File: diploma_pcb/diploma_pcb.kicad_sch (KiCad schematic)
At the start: 15 parts, among them Q1 2SC3356, Q3 2SC3356

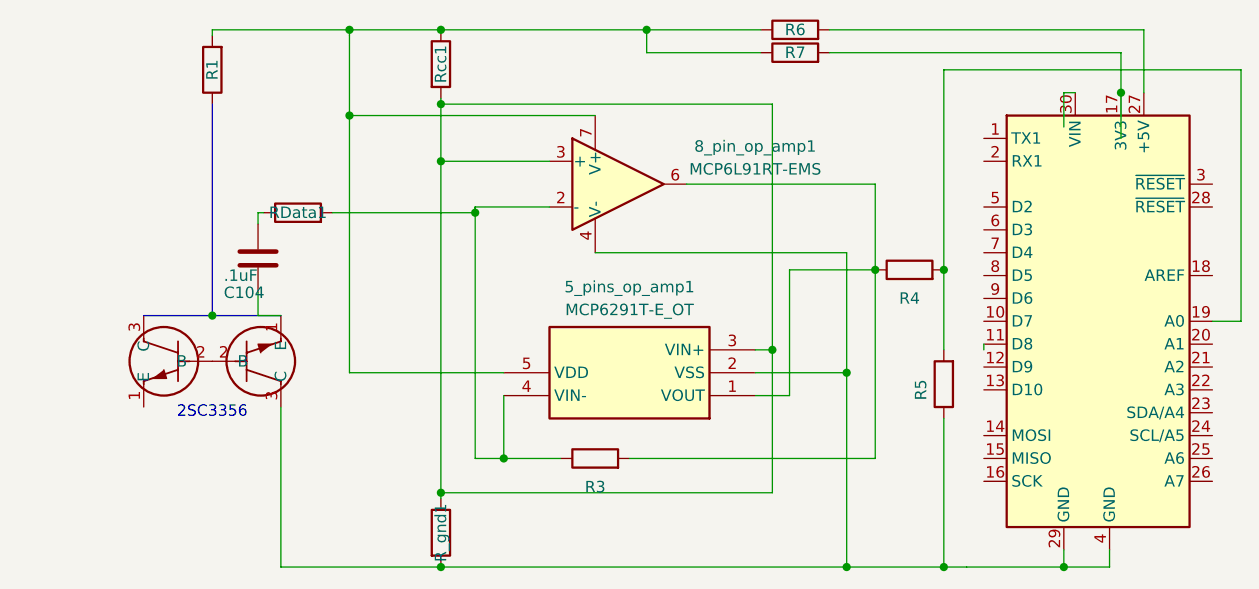
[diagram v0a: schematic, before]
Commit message: with capacitors
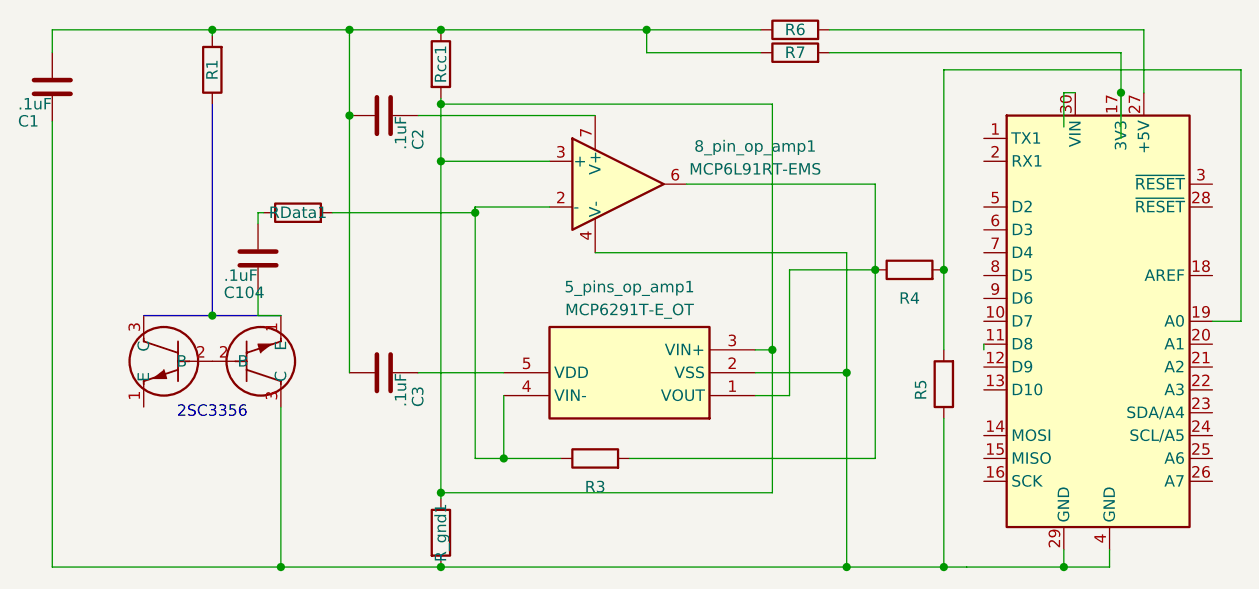
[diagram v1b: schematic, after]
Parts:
- added C1, C2, C3: .1uF, Capacitor_SMD:C_1206_3216Metric_Pad1.33x1.80mm_HandSolder, symbol Device:C
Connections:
- net at 5_pins_op_amp1.2 (VSS), 8_pin_op_amp1.4 (V-), A1.29 (GND)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: now also C1.1
- net at R1.2, R6.1, R7.1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: now also C1.2, C2.2, C3.2; no longer 5_pins_op_amp1.5 (VDD), 8_pin_op_amp1.7 (V+)
- new net: 5_pins_op_amp1.5 (VDD), C3.1
- new net: 8_pin_op_amp1.7 (V+), C2.1
